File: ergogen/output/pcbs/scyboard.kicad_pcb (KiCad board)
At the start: 2 copper layers, 143.9 x 96.5 mm, 54 parts

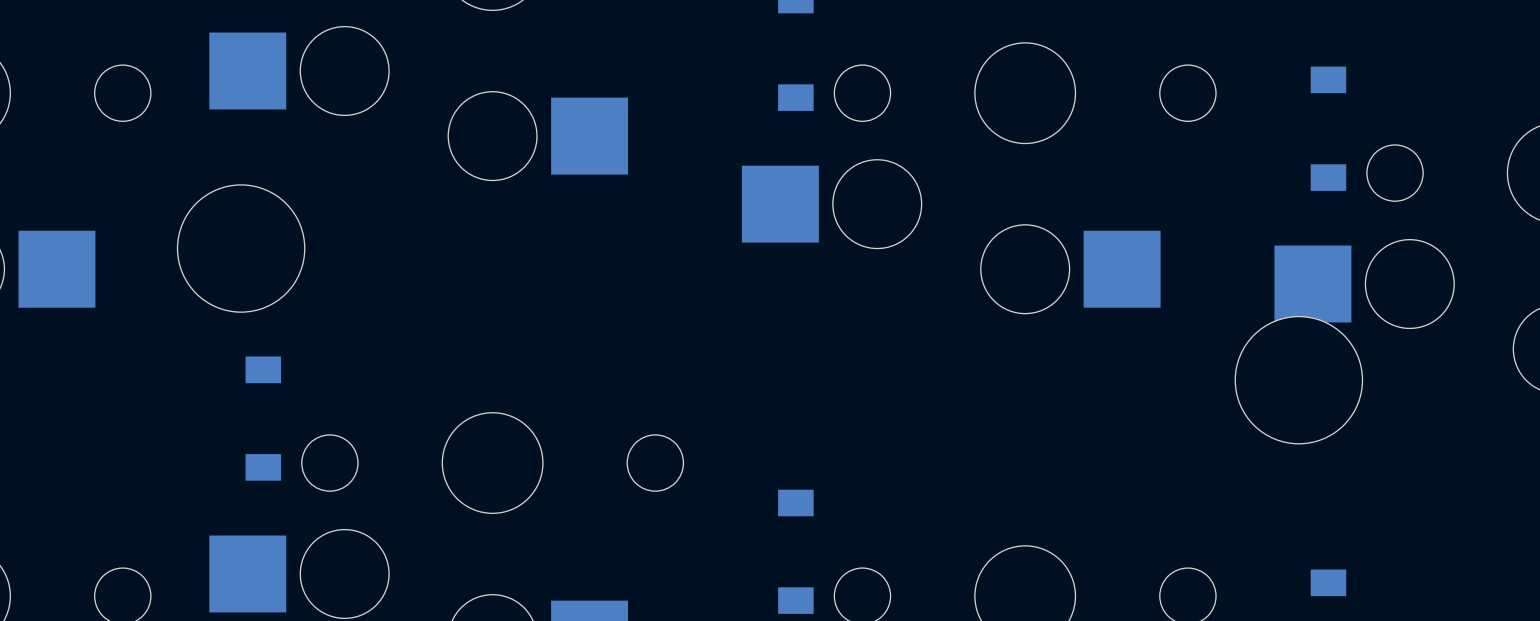
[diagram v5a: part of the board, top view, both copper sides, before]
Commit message: Compile
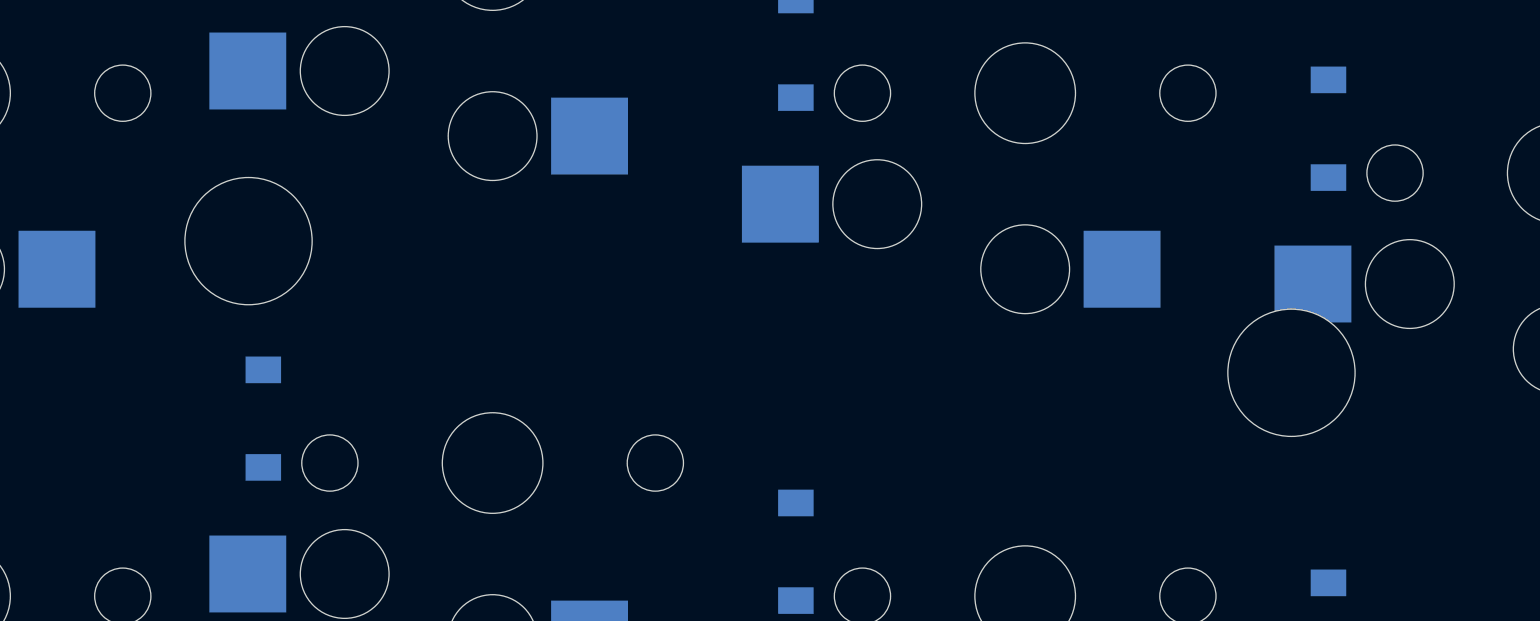
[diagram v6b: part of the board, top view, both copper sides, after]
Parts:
- moved MH4 0.35 mm to (95.8, 57.3)
- moved MH5 0.35 mm to (131.0, 61.8)
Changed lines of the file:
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@@
   (footprint "ceoloide:mounting_hole_npth"
     (layer "F.Cu")
-    (at 95.5 57.56999999999999 0)
+    (at 95.75 57.31999999999999 0)
     (property "Reference" "MH4"
       (at 0 2.55 0)
@@
   (footprint "ceoloide:mounting_hole_npth"
     (layer "F.Cu")
-    (at 131.25 62.019999999999996 0)
+    (at 131 61.769999999999996 0)
     (property "Reference" "MH5"
       (at 0 2.55 0)

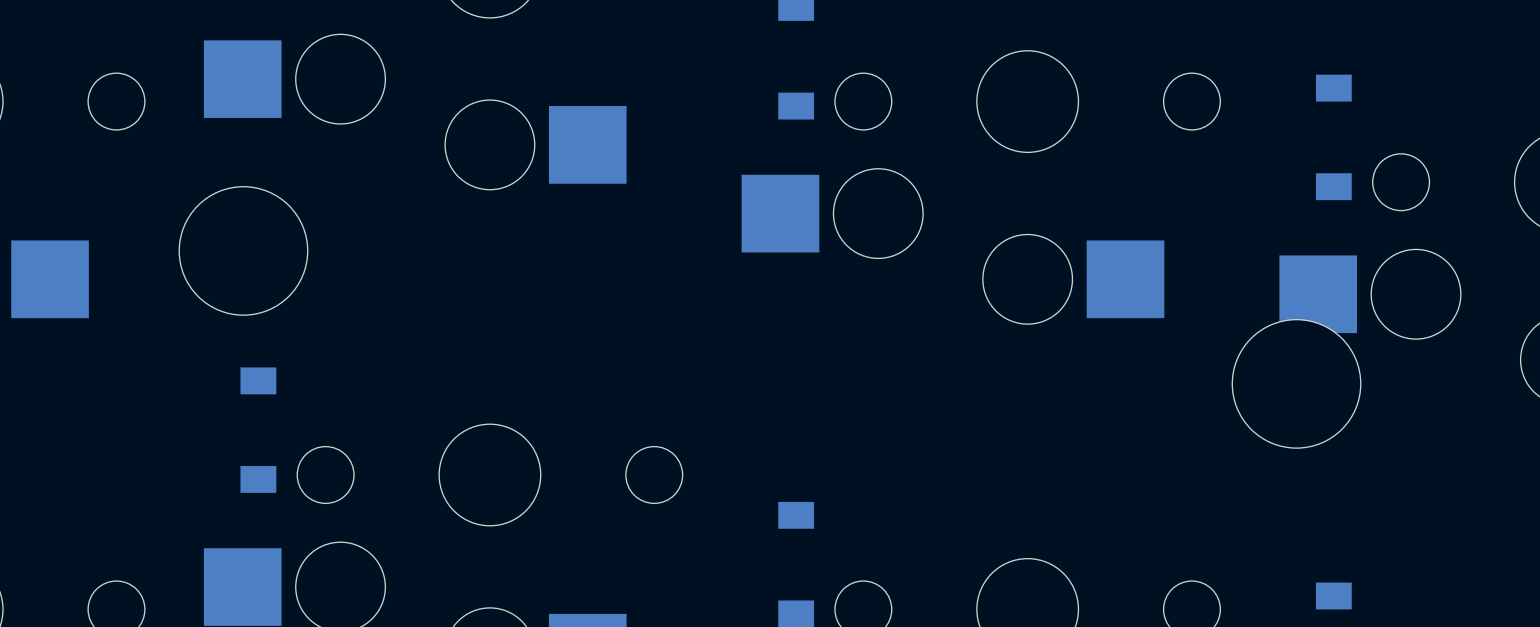
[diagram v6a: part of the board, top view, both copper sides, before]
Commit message: Compile
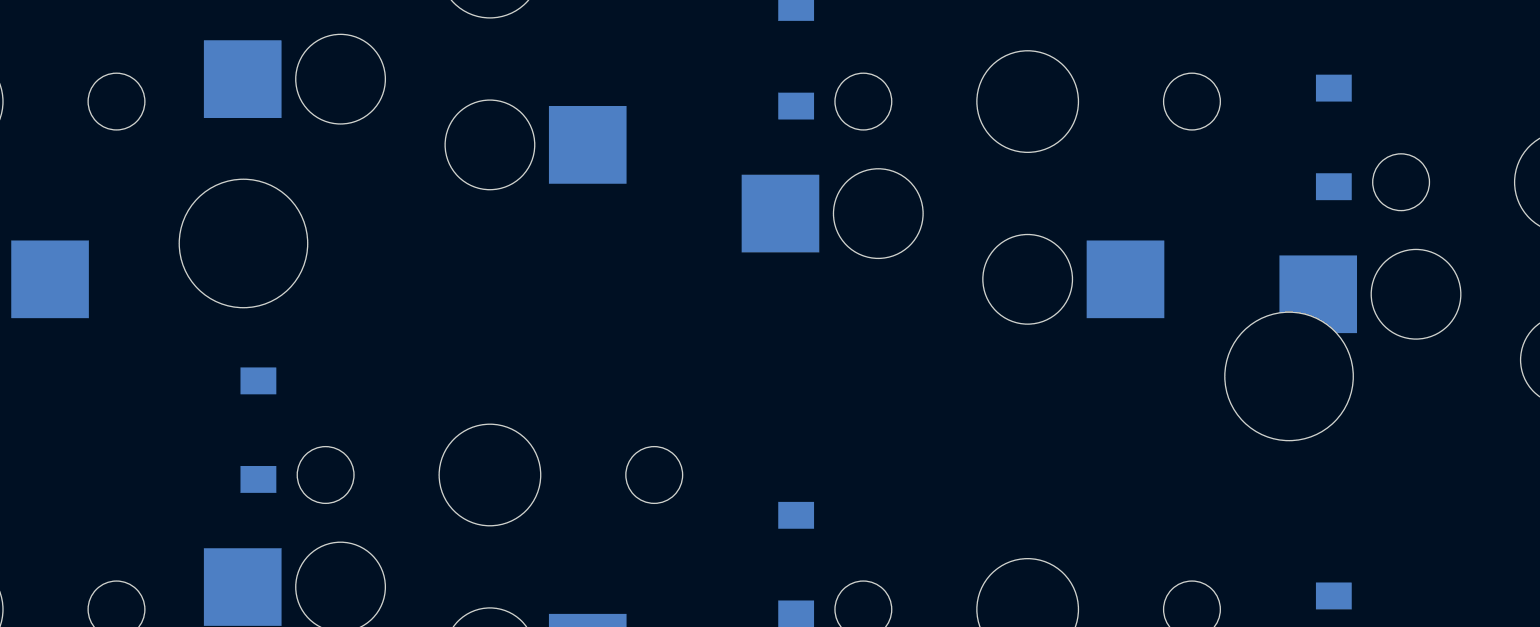
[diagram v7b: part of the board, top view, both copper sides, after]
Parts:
- moved MH5 0.35 mm to (130.8, 61.5)
- moved MH4 0.25 mm to (95.8, 57.1)
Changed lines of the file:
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@@
   (footprint "ceoloide:mounting_hole_npth"
     (layer "F.Cu")
-    (at 95.75 57.31999999999999 0)
+    (at 95.75 57.06999999999999 0)
     (property "Reference" "MH4"
       (at 0 2.55 0)
@@
   (footprint "ceoloide:mounting_hole_npth"
     (layer "F.Cu")
-    (at 131 61.769999999999996 0)
+    (at 130.75 61.519999999999996 0)
     (property "Reference" "MH5"
       (at 0 2.55 0)

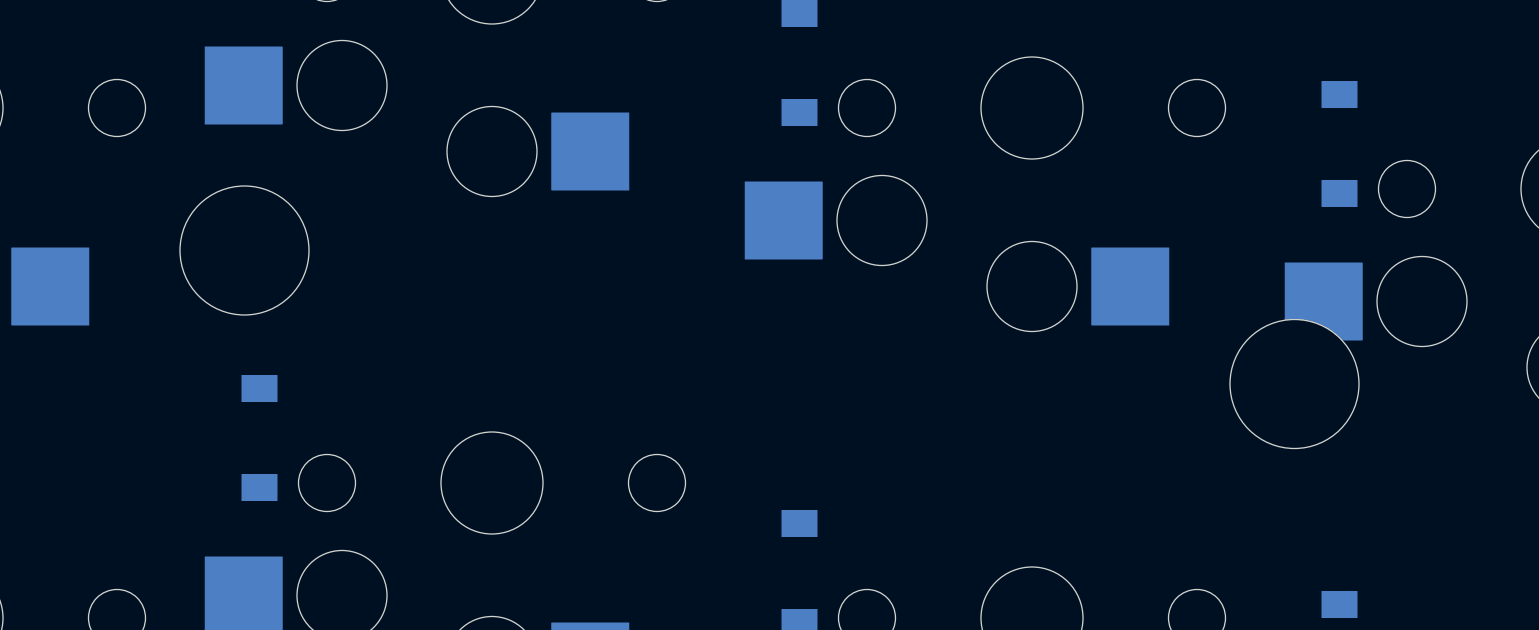
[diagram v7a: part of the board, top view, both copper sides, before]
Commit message: Compile
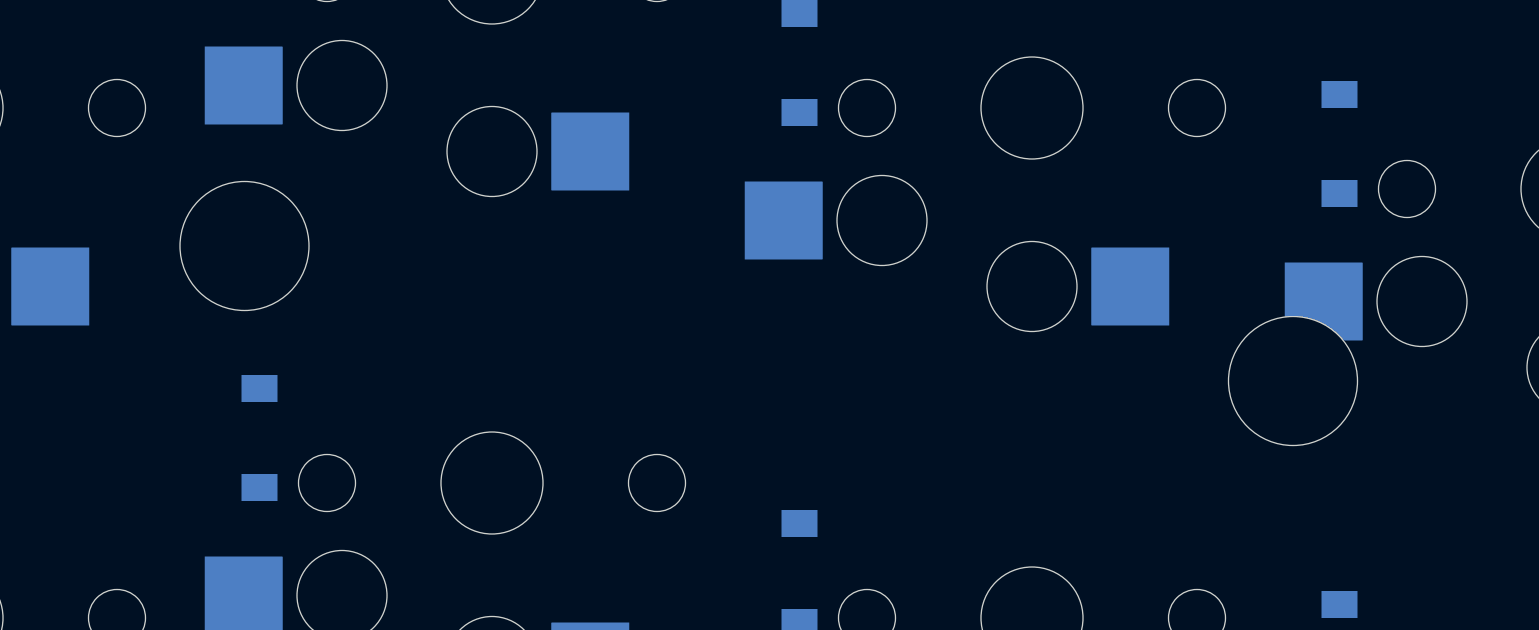
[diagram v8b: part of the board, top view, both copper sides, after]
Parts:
- moved MH4 0.15 mm to (95.8, 56.9)
- moved MH5 0.11 mm to (130.7, 61.4)
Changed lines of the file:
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@@
   (footprint "ceoloide:mounting_hole_npth"
     (layer "F.Cu")
-    (at 95.75 57.06999999999999 0)
+    (at 95.75 56.919999999999995 0)
     (property "Reference" "MH4"
       (at 0 2.55 0)
@@
   (footprint "ceoloide:mounting_hole_npth"
     (layer "F.Cu")
-    (at 130.75 61.519999999999996 0)
+    (at 130.7 61.419999999999995 0)
     (property "Reference" "MH5"
       (at 0 2.55 0)
